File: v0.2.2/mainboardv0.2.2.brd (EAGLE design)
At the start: 33.3 x 29.2 mm, 17 parts, among them U1 BC127, Y1 MHz

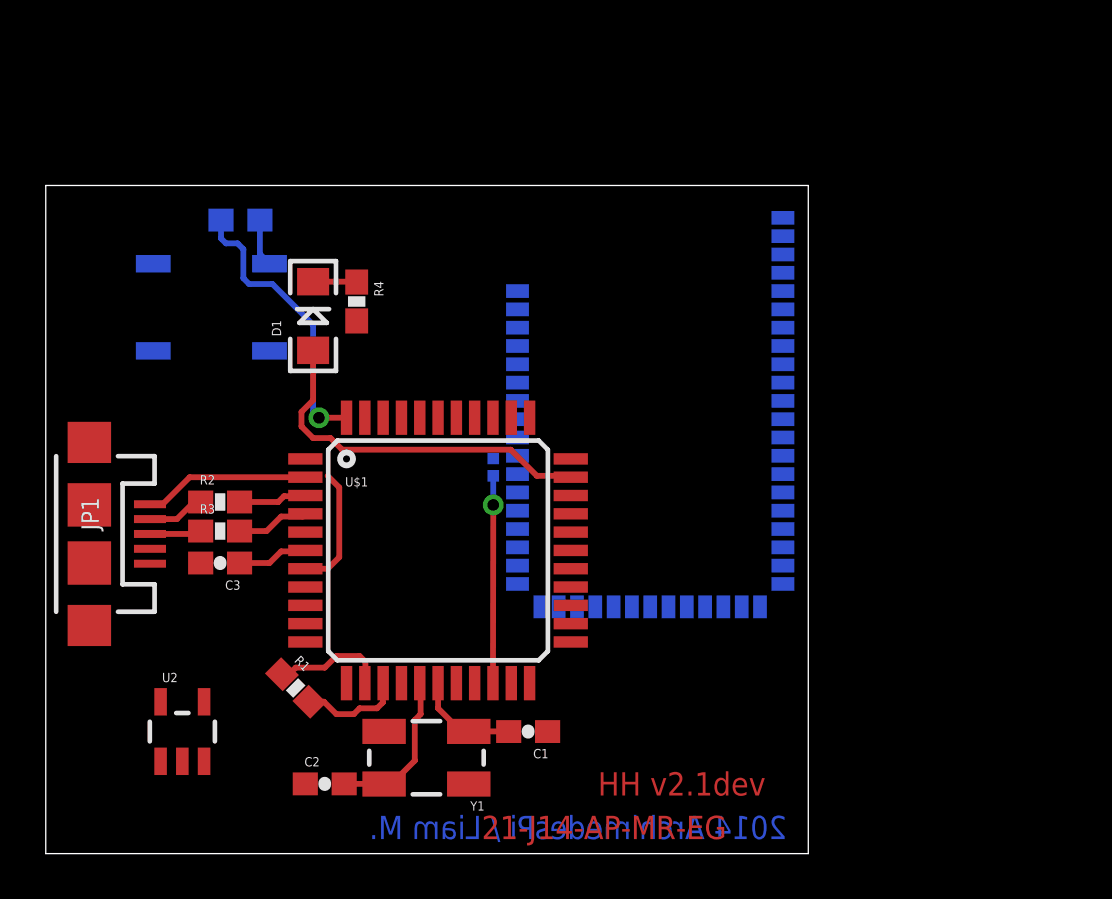
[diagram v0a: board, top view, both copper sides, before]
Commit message: Begin the routing
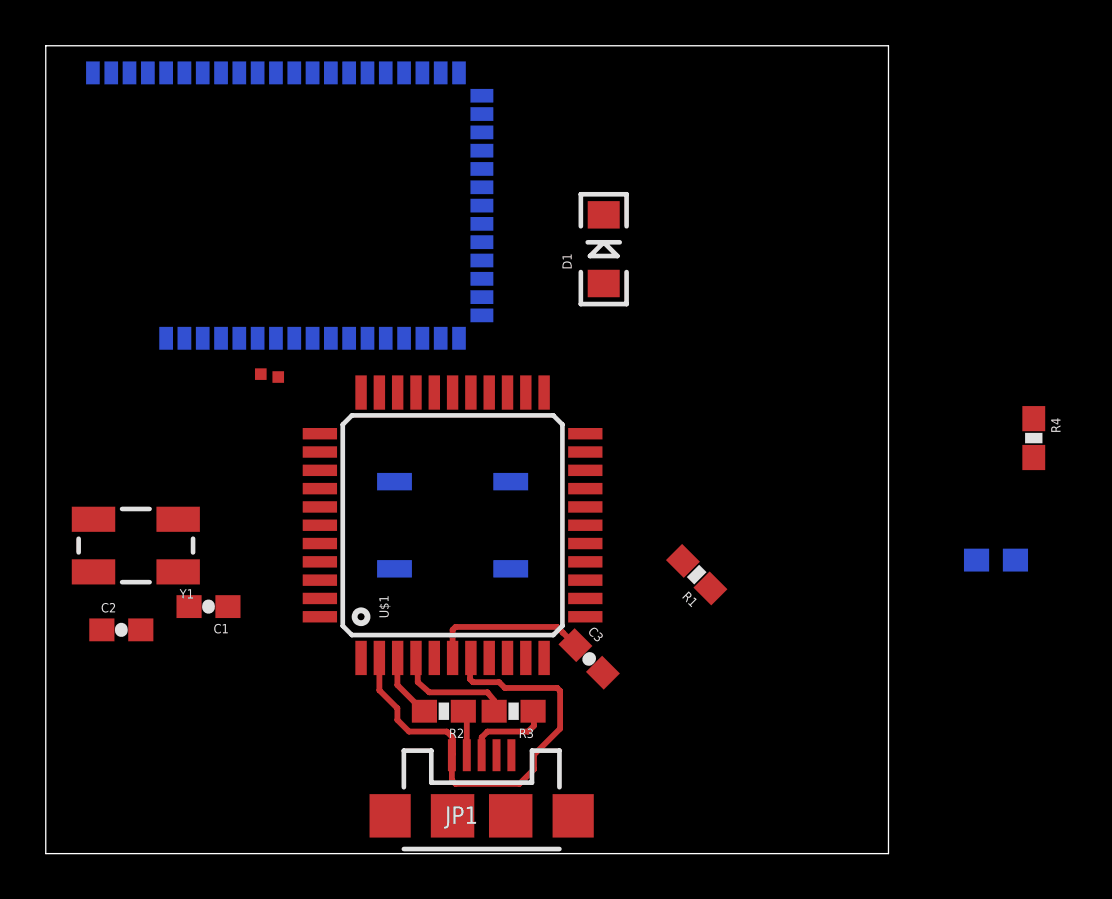
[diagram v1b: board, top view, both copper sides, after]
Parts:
- removed U2: (no value), SparkFun-PowerIC:SOT23-5
- moved R5 36.2 mm to (41.5, 12.8)
- moved R4 30.2 mm to (43.2, 18.2)
- moved JP1 21.1 mm to (19.1, 1.65), turned to 0 degrees
- moved U1 18.4 mm to (10.2, 28.3), turned to 270 degrees
- moved R1 18.2 mm to (28.4, 12.2), turned to 135 degrees
- moved C3 16.7 mm to (23.7, 8.51), turned to 315 degrees
- moved Y1 15.7 mm to (3.94, 13.5)
- moved R3 15.1 mm to (20.4, 6.22), turned to 180 degrees
- moved C1 15.0 mm to (7.11, 10.8)
- moved S1 14.2 mm to (17.8, 14.4)
- moved R2 13.4 mm to (17.4, 6.22), turned to 180 degrees
- moved D1 13.0 mm to (24.4, 26.4)
- moved C2 11.2 mm to (3.30, 9.78)
- moved TP2 11.1 mm to (9.40, 21.0), flipped to the top
- moved TP1 10.0 mm to (10.2, 20.8), flipped to the top
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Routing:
- net +3V3: track 17.0 -> 0.00 mm, vias 1 -> 0
- net LED: track 16.2 -> 0.00 mm
- net N$9: track 9.06 -> 0.00 mm, vias 1 -> 0
- net VCC/2: track 12.7 -> 20.6 mm
- net N$3: track 7.02 -> 0.00 mm
- net N$1: track 5.03 -> 0.00 mm
- net N$2: track 4.61 -> 0.00 mm
- net N$4: track 3.10 -> 6.98 mm
- net N$6: track 2.08 -> 0.00 mm
- net D+: track 3.19 -> 5.23 mm
- net N$5: track 1.91 -> 0.00 mm
- net N$8: track 2.27 -> 3.93 mm
- net N$7: track 2.52 -> 1.98 mm
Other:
- board size 33.3 x 29.2 mm -> 36.8 x 35.3 mm
- board text removed: "2014 ArchimedesPi / Liam M."
- board text removed: "21-J14-AP-MR-EG"
- board text removed: "HH v2.1dev"
